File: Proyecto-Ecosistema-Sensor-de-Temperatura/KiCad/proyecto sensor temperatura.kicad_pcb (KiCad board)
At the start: 2 copper layers, 30.5 x 77.5 mm, 8 parts

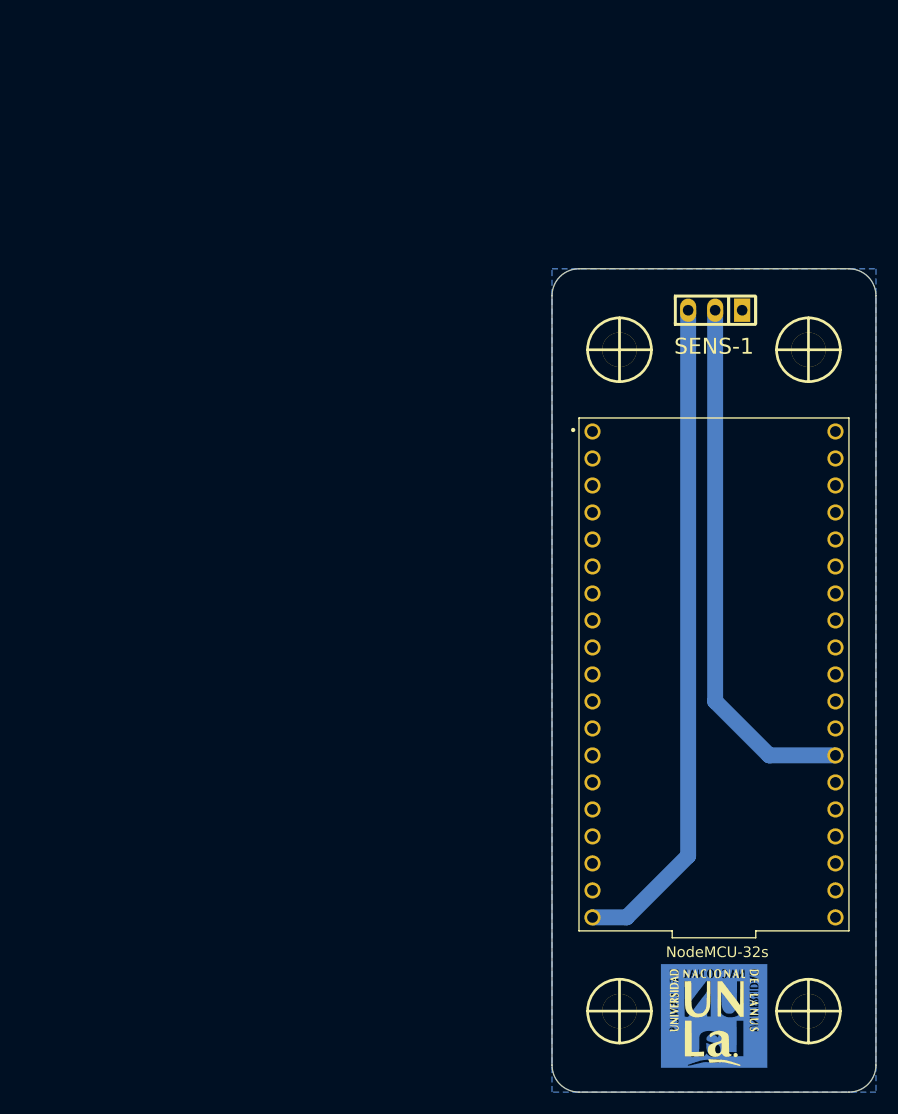
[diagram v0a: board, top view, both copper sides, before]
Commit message: Importar contenido de proyecto-sensor-temperatura-humedad a main
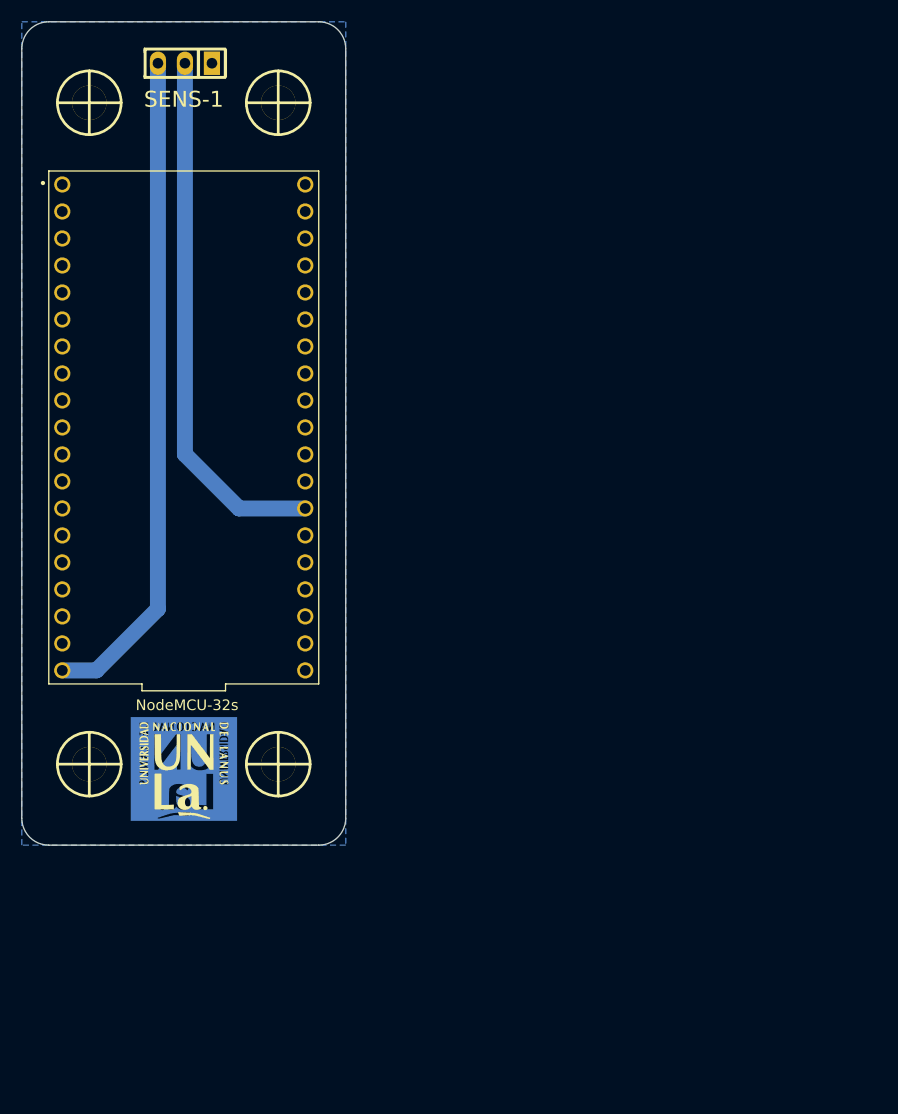
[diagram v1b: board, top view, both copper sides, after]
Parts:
- moved H1 55.0 mm to (82.2, 60.6)
- moved H2 55.0 mm to (82.2, 122.8)
- moved H4 55.0 mm to (64.4, 122.8)
- moved Logo UNLa 55.0 mm to (73.3, 123.3)
- moved Micro_controlador1 55.0 mm to (73.3, 91.1)
- moved UNLa Logo Invertido 55.0 mm to (73.3, 123.3)
- moved H3 55.0 mm to (64.4, 60.6)
- moved SENS-1 55.0 mm to (73.4, 56.9)
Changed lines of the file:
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@@
     (thickness 1.6)
   )
-  (paper "A4")
+  (paper "A5" portrait)
   (layers
     (0 "F.Cu" signal)
@@
       (sketchpadsonfab false)
       (subtractmaskfromsilk false)
-      (outputformat 1)
+      (outputformat 4)
       (mirror false)
-      (drillshape 1)
+      (drillshape 0)
       (scaleselection 1)
-      (outputdirectory "")
+      (outputdirectory "./")
     )
   )
@@
   (net 36 "unconnected-(Micro_controlador1-Pad37)")
   (footprint "EESTN5:Separador_M3_5mm" (layer "F.Cu")
-    (at 132.08 83.82)
+    (at 82.191 60.581)
     (descr "Separador M3 5mm de alto")
     (property "Sheetfile" "proyecto sensor temperatura.kicad_sch")
@@
   )
   (footprint "EESTN5:Separador_M3_5mm" (layer "F.Cu")
-    (at 132.08 146.05)
+    (at 82.191 122.811)
     (descr "Separador M3 5mm de alto")
     (property "Sheetfile" "proyecto sensor temperatura.kicad_sch")
@@
   )
   (footprint "NODEMCU-32S:MODULE_NODEMCU-32S" (layer "F.Cu")
-    (at 123.19 114.369)
+    (at 73.301 91.13)
     (property "Sheetfile" "proyecto sensor temperatura.kicad_sch")
     (property "Sheetname" "")
@@
   )
   (footprint "UNLaLibreria:logoUnlaFootprintNoNegativeInvertida" (layer "F.Cu")
-    (at 123.19 146.5)
+    (at 73.301 123.261)
     (attr board_only exclude_from_pos_files exclude_from_bom)
     (fp_text reference "UNLa Logo Invertido" (at 0 -7.62) (layer "F.SilkS") hide
@@
   )
   (footprint "EESTN5:Pin_Header_3" (layer "F.Cu")
-    (at 123.3 80.1 180)
+    (at 73.411 56.861 180)
     (descr "Pin socket 3 pin")
     (tags "CONN DEV")
@@
   )
   (footprint "EESTN5:Separador_M3_5mm" (layer "F.Cu")
-    (at 114.3 146.05)
+    (at 64.411 122.811)
     (descr "Separador M3 5mm de alto")
     (property "Sheetfile" "proyecto sensor temperatura.kicad_sch")
@@
   )
   (footprint "UNLaLibreria:logoUnlaFootprint" (layer "F.Cu")
-    (at 123.19 146.5)
+    (at 73.301 123.261)
     (attr board_only exclude_from_pos_files exclude_from_bom)
     (fp_text reference "Logo UNLa" (at 31.75 10.16) (layer "F.SilkS") hide
@@
   )
   (footprint "EESTN5:Separador_M3_5mm" (layer "F.Cu")
-    (at 114.3 83.82)
+    (at 64.411 60.581)
     (descr "Separador M3 5mm de alto")
     (property "Sheetfile" "proyecto sensor temperatura.kicad_sch")
@@
     )
   )
-  (gr_arc (start 107.950001 78.740001) (mid 108.693949 76.943949) (end 110.490001 76.200001) (layer "Edge.Cuts") (width 0.1))
-  (gr_line (start 135.889999 76.200001) (end 110.490001 76.200001) (layer "Edge.Cuts") (width 0.1))
-  (gr_arc (start 110.49 153.67) (mid 108.693949 152.926051) (end 107.95 151.13) (layer "Edge.Cuts") (width 0.1))
-  (gr_line (start 110.49 153.67) (end 135.889999 153.669999) (layer "Edge.Cuts") (width 0.1))
-  (gr_arc (start 138.429999 151.129999) (mid 137.686051 152.926051) (end 135.889999 153.669999) (layer "Edge.Cuts") (width 0.1))
-  (gr_arc (start 135.889999 76.200001) (mid 137.686051 76.943949) (end 138.429999 78.740001) (layer "Edge.Cuts") (width 0.1))
-  (gr_line (start 138.429999 151.129999) (end 138.429999 78.740001) (layer "Edge.Cuts") (width 0.1))
-  (gr_line (start 107.950001 78.740001) (end 107.95 151.13) (layer "Edge.Cuts") (width 0.1))
-  (segment (start 120.76 80.1) (end 120.76 131.44) (width 1.5) (layer "B.Cu") (net 18))
-  (segment (start 114.971 137.229) (end 111.76 137.229) (width 1.5) (layer "B.Cu") (net 18))
-  (segment (start 120.76 131.44) (end 114.971 137.229) (width 1.5) (layer "B.Cu") (net 18))
-  (segment (start 123.3 80.1) (end 123.3 116.9) (width 1.5) (layer "B.Cu") (net 25))
-  (segment (start 123.3 116.9) (end 128.389 121.989) (width 1.5) (layer "B.Cu") (net 25))
-  (segment (start 128.389 121.989) (end 134.62 121.989) (width 1.5) (layer "B.Cu") (net 25))
+  (gr_arc (start 58.061001 55.501001) (mid 58.804949 53.704949) (end 60.601001 52.961001) (layer "Edge.Cuts") (width 0.1))
+  (gr_line (start 86.000999 52.961001) (end 60.601001 52.961001) (layer "Edge.Cuts") (width 0.1))
+  (gr_arc (start 60.601 130.431) (mid 58.804949 129.687051) (end 58.061 127.891) (layer "Edge.Cuts") (width 0.1))
+  (gr_line (start 60.601 130.431) (end 86.000999 130.430999) (layer "Edge.Cuts") (width 0.1))
+  (gr_arc (start 88.540999 127.890999) (mid 87.797051 129.687051) (end 86.000999 130.430999) (layer "Edge.Cuts") (width 0.1))
+  (gr_arc (start 86.000999 52.961001) (mid 87.797051 53.704949) (end 88.540999 55.501001) (layer "Edge.Cuts") (width 0.1))
+  (gr_line (start 88.540999 127.890999) (end 88.540999 55.501001) (layer "Edge.Cuts") (width 0.1))
+  (gr_line (start 58.061001 55.501001) (end 58.061 127.891) (layer "Edge.Cuts") (width 0.1))
+  (segment (start 70.871 56.861) (end 70.871 108.201) (width 1.5) (layer "B.Cu") (net 18))
+  (segment (start 65.082 113.99) (end 61.871 113.99) (width 1.5) (layer "B.Cu") (net 18))
+  (segment (start 70.871 108.201) (end 65.082 113.99) (width 1.5) (layer "B.Cu") (net 18))
+  (segment (start 73.411 56.861) (end 73.411 93.661) (width 1.5) (layer "B.Cu") (net 25))
+  (segment (start 73.411 93.661) (end 78.5 98.75) (width 1.5) (layer "B.Cu") (net 25))
+  (segment (start 78.5 98.75) (end 84.731 98.75) (width 1.5) (layer "B.Cu") (net 25))
   (zone (net 30) (net_name "GND") (layer "B.Cu") (hatch edge 0.508)
     (connect_pads yes (clearance 0.8))
@@
     (polygon
       (pts
-        (xy 138.43 153.67)
-        (xy 107.95 153.67)
-        (xy 107.95 76.2)
-        (xy 138.43 76.2)
+        (xy 88.541 130.431)
+        (xy 58.061 130.431)
+        (xy 58.061 52.961)
+        (xy 88.541 52.961)
       )
     )
@@
     (polygon
       (pts
-        (xy 128.77 152)
-        (xy 117.61 152)
-        (xy 117.61 141.09)
-        (xy 128.77 141.09)
+        (xy 78.881 128.761)
+        (xy 67.721 128.761)
+        (xy 67.721 117.851)
+        (xy 78.881 117.851)
       )
     )
